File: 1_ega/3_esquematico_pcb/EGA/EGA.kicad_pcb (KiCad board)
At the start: 2 copper layers, 100 x 100 mm, 46 parts, among them J1 Entrada de 12V, J10 M1, J11 M2, J12 IN1 IN2 EN, J13 OUT, J14 I2C, J15 12, J16 5, J17 UART, J18 SW DT CLK, J19 SPI, J2 Motor, J20 LEDS, J21 BOTONES, J22 GND, J23 GND, J24 GND, J25 GND, J3 Pantalla LCD, J4 Memoria SD, J5 Sensor IR, J6 Encoder, J7 RTC, J8 EGB_I2C, J9 EGB_UART, SW1 Sentido, SW2 Calibrar, U1 L7805, U2 L298N

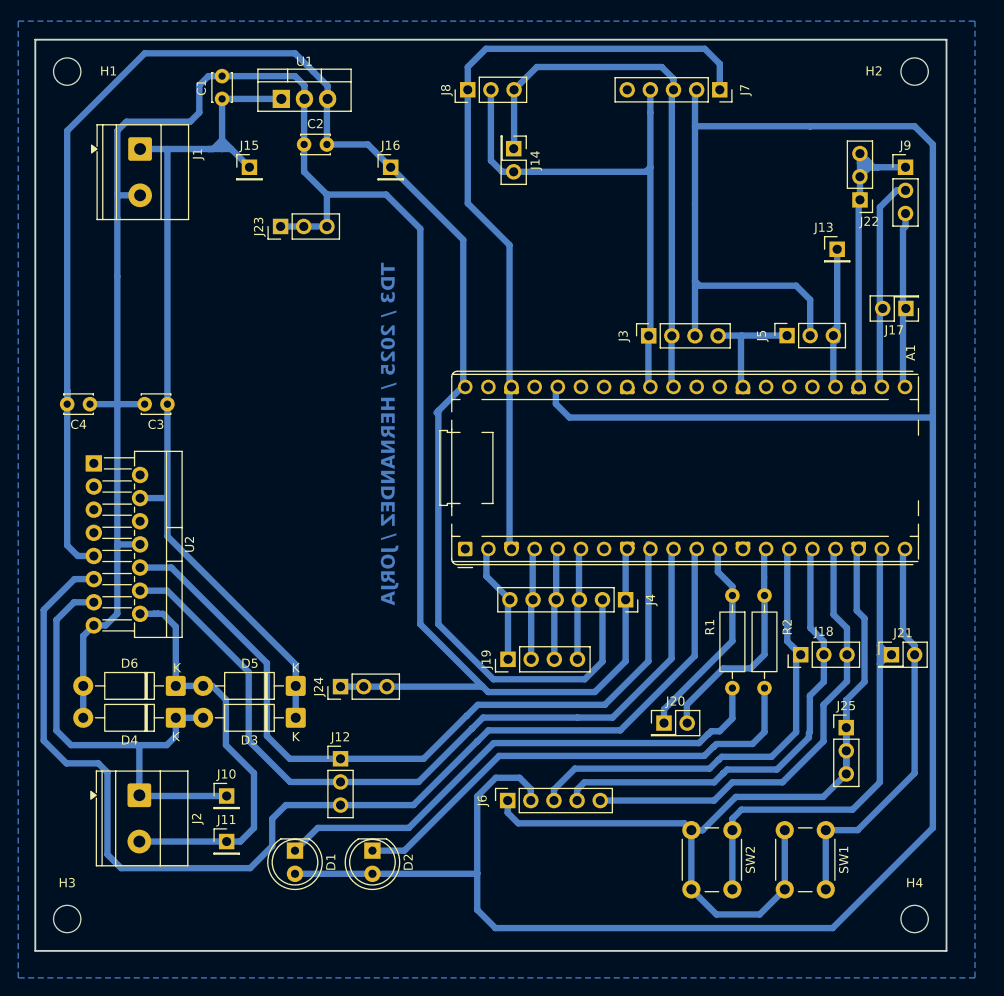
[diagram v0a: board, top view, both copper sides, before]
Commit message: Archivo de KiCad final
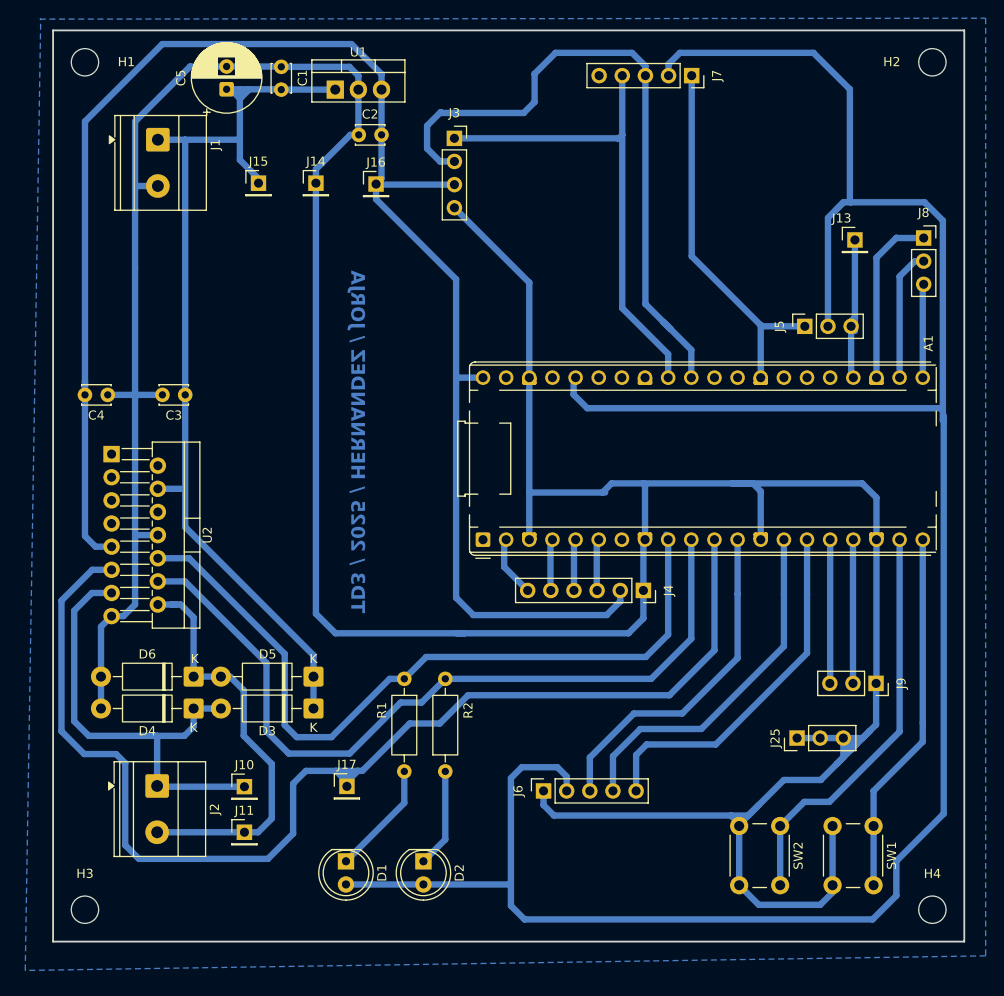
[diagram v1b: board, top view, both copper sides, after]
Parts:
- removed J12: IN1 IN2 EN, Connector_PinHeader_2.54mm:PinHeader_1x03_P2.54mm_Vertical
- removed J18: SW DT CLK, Connector_PinHeader_2.54mm:PinHeader_1x03_P2.54mm_Vertical
- removed J19: SPI, Connector_PinHeader_2.54mm:PinHeader_1x04_P2.54mm_Vertical
- removed J20: LEDS, Connector_PinHeader_2.54mm:PinHeader_2x01_P2.54mm_Vertical
- removed J21: BOTONES, Connector_PinHeader_2.54mm:PinHeader_2x01_P2.54mm_Vertical
- removed J22, J23, J24: GND, Connector_PinHeader_2.54mm:PinHeader_1x03_P2.54mm_Vertical
- added C5: 100uF, Capacitor_THT:CP_Radial_D7.5mm_P2.50mm, F.Cu at (116.5, 52.5)
- C1: value 0,22uF -> 0,1uF
- J14: value I2C -> GND; footprint Connector_PinHeader_2.54mm:PinHeader_2x01_P2.54mm_Vertical -> Connector_PinHeader_2.54mm:PinHeader_1x01_P2.54mm_Vertical
- J17: value UART -> EnB; footprint Connector_PinHeader_2.54mm:PinHeader_2x01_P2.54mm_Vertical -> Connector_PinHeader_2.54mm:PinHeader_1x01_P2.54mm_Vertical
- J8, J9: footprint Connector_PinHeader_2.54mm:PinHeader_1x03_P2.54mm_Vertical -> Connector_PinSocket_2.54mm:PinSocket_1x03_P2.54mm_Vertical
- moved J17 80.7 mm to (129.7, 129.0), turned to 0 degrees
- moved J9 56.7 mm to (187.7, 117.7), turned to -90 degrees
- moved J8 52.6 mm to (192.9, 68.8), turned to 0 degrees
- moved R1 37.1 mm to (135.9, 117.2)
- moved R2 36.2 mm to (140.4, 127.3)
- moved J3 30.4 mm to (141.4, 57.9), turned to 0 degrees
- moved J14 22.0 mm to (126.2, 62.8), turned to 0 degrees
- moved C1 6.57 mm to (122.5, 52.5)
- moved C2 6.09 mm to (130.9, 57.5)
- moved U1 6.00 mm to (128.4, 52.5)
- moved D1 5.72 mm to (129.6, 137.2)
- moved D2 5.72 mm to (138.1, 137.2)
- moved J25 5.52 mm to (179.1, 123.7), turned to 90 degrees
- moved SW1 5.26 mm to (187.4, 133.3)
- moved SW2 5.26 mm to (177.2, 133.3)
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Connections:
- net BC renamed Net-(A1-GPIO14)
- net BS renamed Net-(A1-GPIO15)
- A1 pad 12: LEDH -> SW
- A1 pad 14: LEDA -> DT
- A1 pad 15: SW -> CLK
- A1 pad 16: DT -> UART TX
- A1 pad 17: CLK -> UART RX
- A1 pad 21: UART TX -> SDA_EGB
- A1 pad 22: UART RX -> SCL_EGB
- J14 pad 1: SDA -> GND
- J17 pad 1: UART TX -> EnB
- J3 pad 3: +3.3V -> +5V
- J8 pad 2: SCL -> SCL_EGB
- J8 pad 3: SDA -> SDA_EGB
- R1 pad 1: LEDH -> IN3
- R2 pad 2: LEDA -> IN4
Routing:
- net Net-(D1-K): track 57.3 -> 12.9 mm
- net Net-(D2-K): track 53.2 -> 10.9 mm
- net LEDA: track 24.5 -> 0.00 mm
- net LEDH: track 23.5 -> 0.00 mm
- net +3.3V: track 287.2 -> 267.9 mm
- net SW: track 52.4 -> 37.9 mm
- net SCL_EGB: track 0.00 -> 14.5 mm
- net SDA: track 59.4 -> 73.3 mm
- net DT: track 51.1 -> 39.3 mm
- net Net-(A1-GPIO14): track 55.7 -> 45.0 mm
- net SDA_EGB: track 0.00 -> 10.7 mm
- net CLK: track 50.1 -> 39.8 mm
- net GND: track 475.2 -> 483.1 mm
- net EnB: track 127.0 -> 134.4 mm
- net +12V: track 99.1 -> 106.4 mm
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
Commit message: Cambio en R1 y R2
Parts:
- R1, R2: value 330 -> 180
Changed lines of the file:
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@@
 			)
 		)
-		(property "Value" "330"
+		(property "Value" "180"
 			(at 5.08 2.37 90)
 			(layer "F.Fab")
@@
 			)
 		)
-		(property "Value" "330"
+		(property "Value" "180"
 			(at 5.08 2.37 90)
 			(layer "F.Fab")
